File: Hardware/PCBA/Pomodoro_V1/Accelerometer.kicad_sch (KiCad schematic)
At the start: 8 parts, among them U2 LIS2HH12

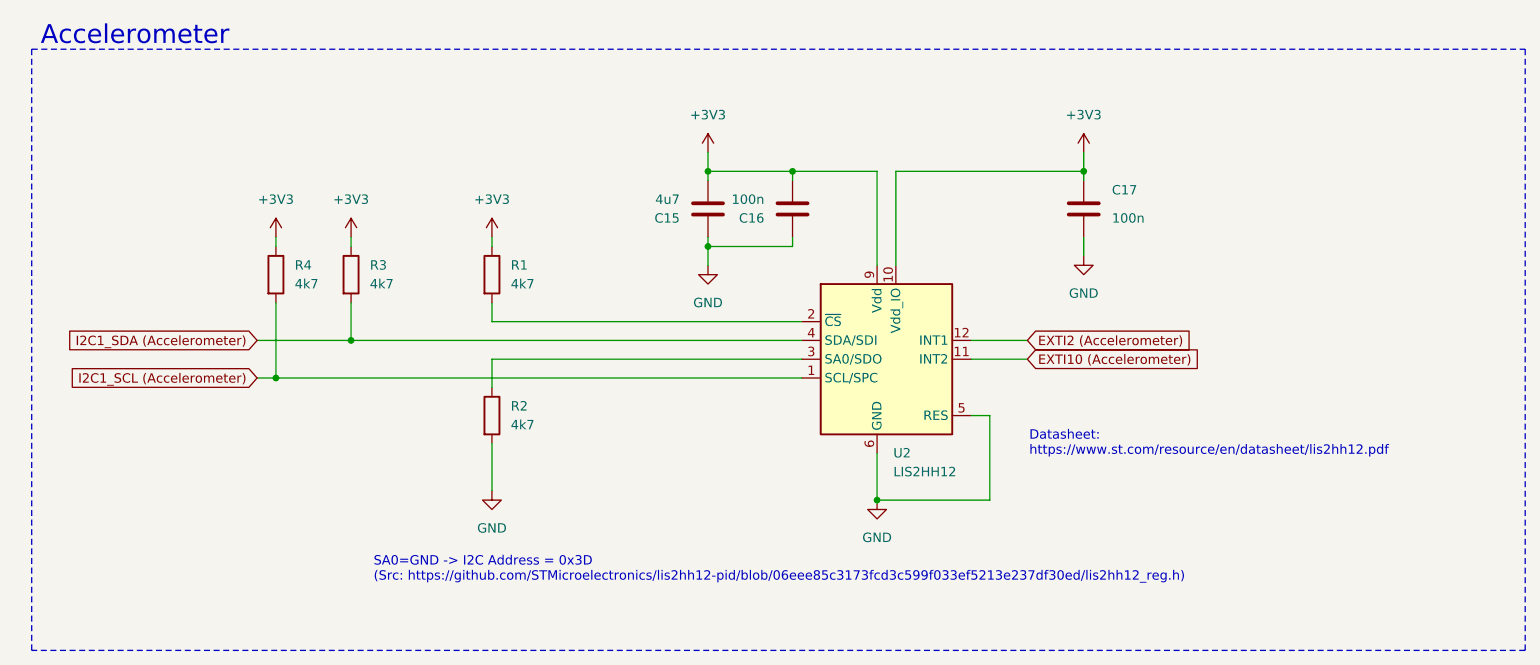
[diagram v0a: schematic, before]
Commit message: Finalized the schematic, First Draft of the finished Layout
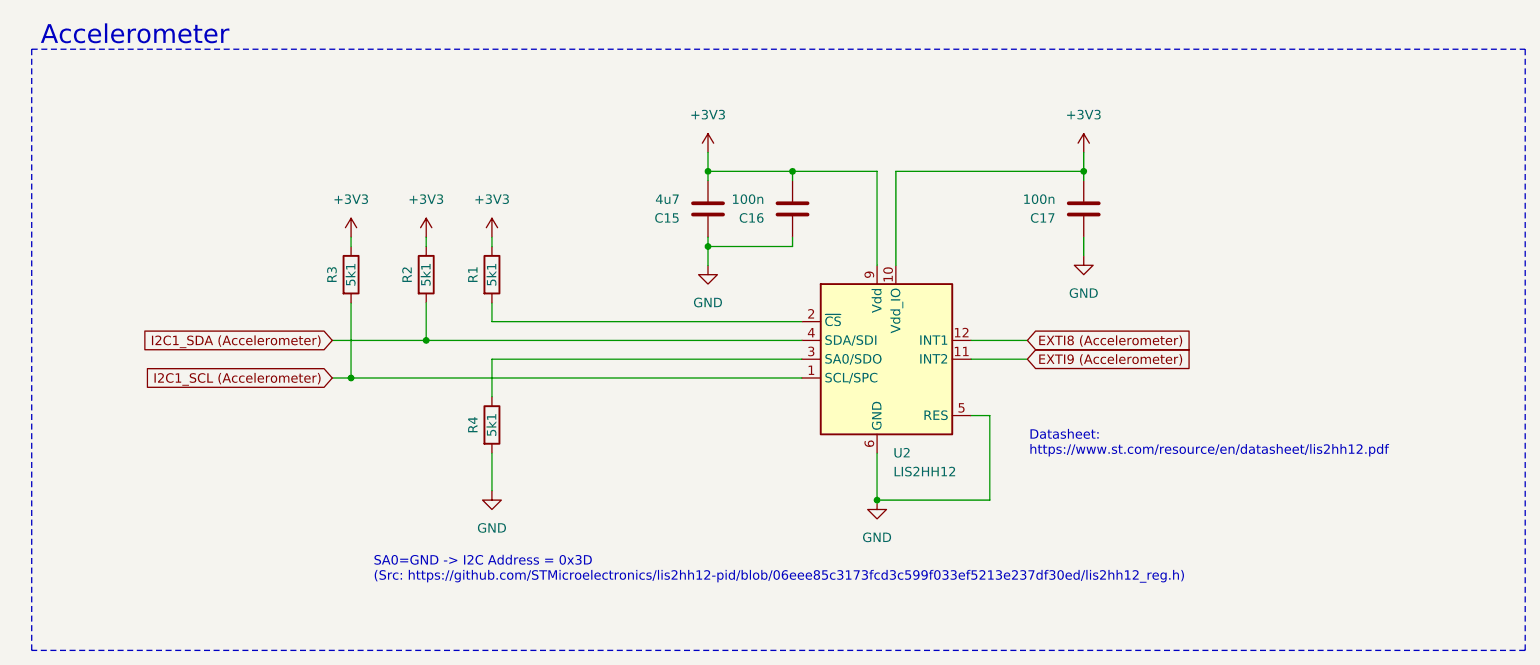
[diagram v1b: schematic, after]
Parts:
- C15, C16, C17: footprint (none) -> Capacitor_SMD:C_0805_2012Metric
- R1, R2, R3, R4: value 4k7 -> 5k1; footprint (none) -> Resistor_SMD:R_0805_2012Metric; Part ID (none) -> CR0805-FX-5101ELF
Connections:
- net +3V3: now also C17.2, R2.1; no longer C17.1, R4.1
- net GND: now also C17.1, R4.2; no longer C17.2, R2.2
- net I2C1_SCL (Accelerometer): now also R3.2; no longer R4.2
- net I2C1_SDA (Accelerometer): now also R2.2; no longer R3.2
- net at U2.3 (SA0/SDO): now also R4.1; no longer R2.1
- net EXTI10 (Accelerometer) renamed EXTI9 (Accelerometer)
- net EXTI2 (Accelerometer) renamed EXTI8 (Accelerometer)
